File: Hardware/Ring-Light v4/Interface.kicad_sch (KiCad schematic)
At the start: 15 parts, among them J2 USB_B_Micro, U37 CP2102N-A02-GQFN20R

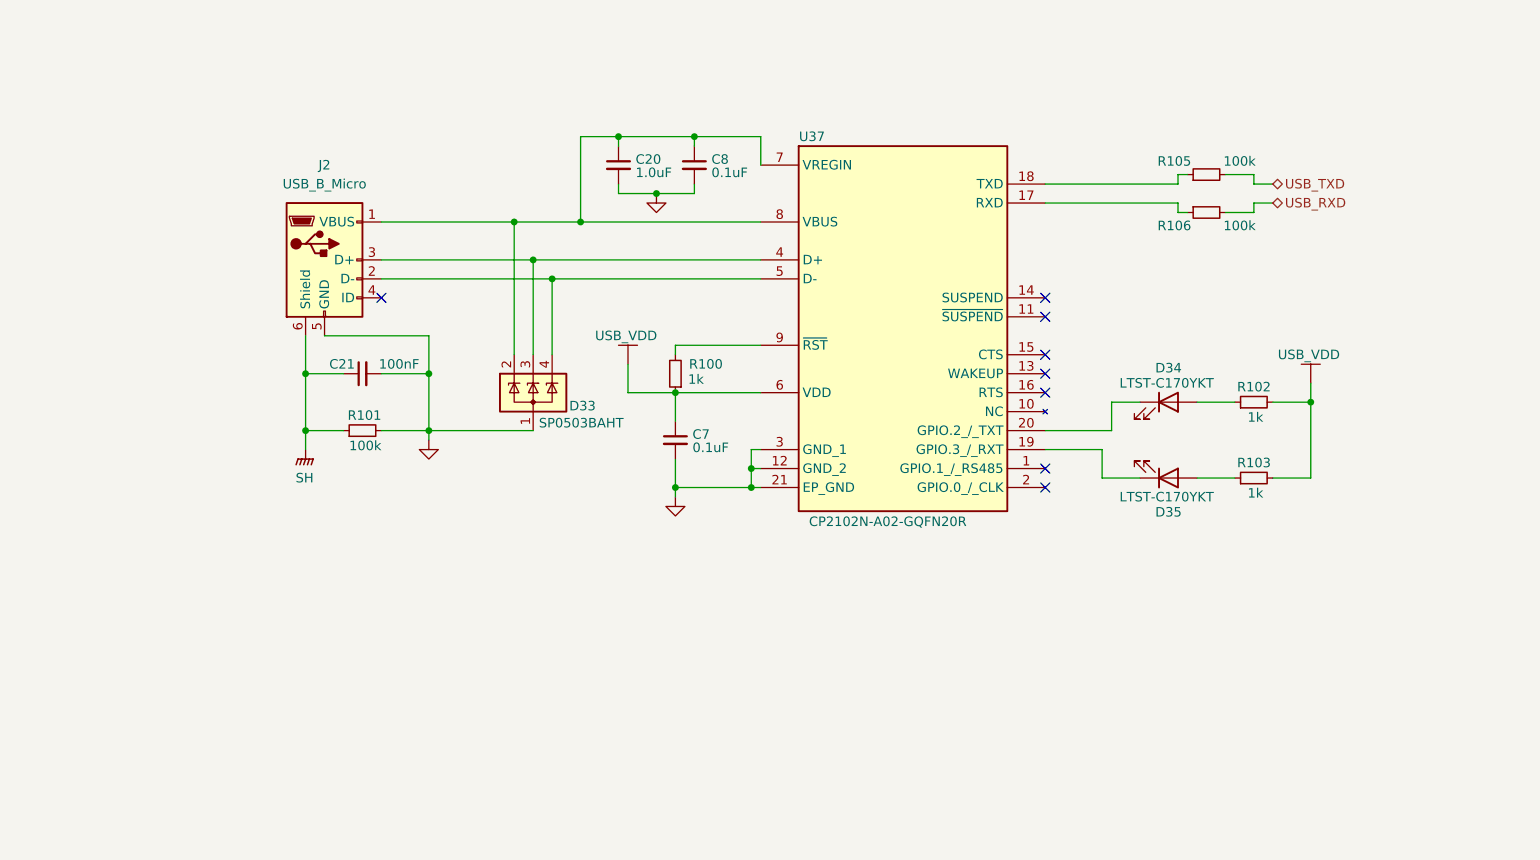
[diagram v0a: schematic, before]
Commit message: m
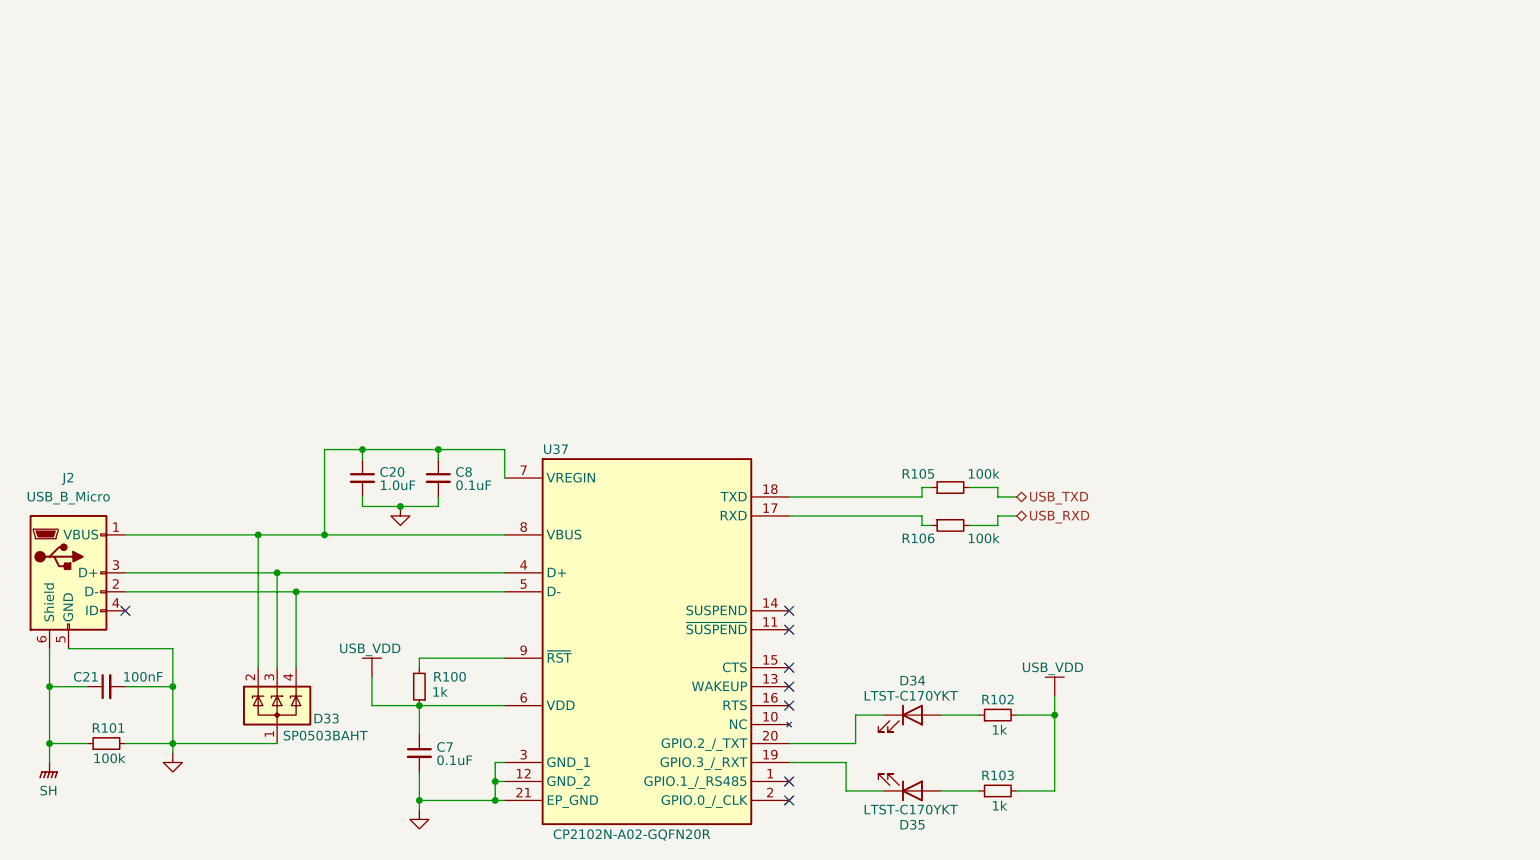
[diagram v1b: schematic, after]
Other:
- moved on the sheet: C20, C21, C7, C8, D33, D34, D35, J2, R100, R101, R102, R103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

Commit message: m
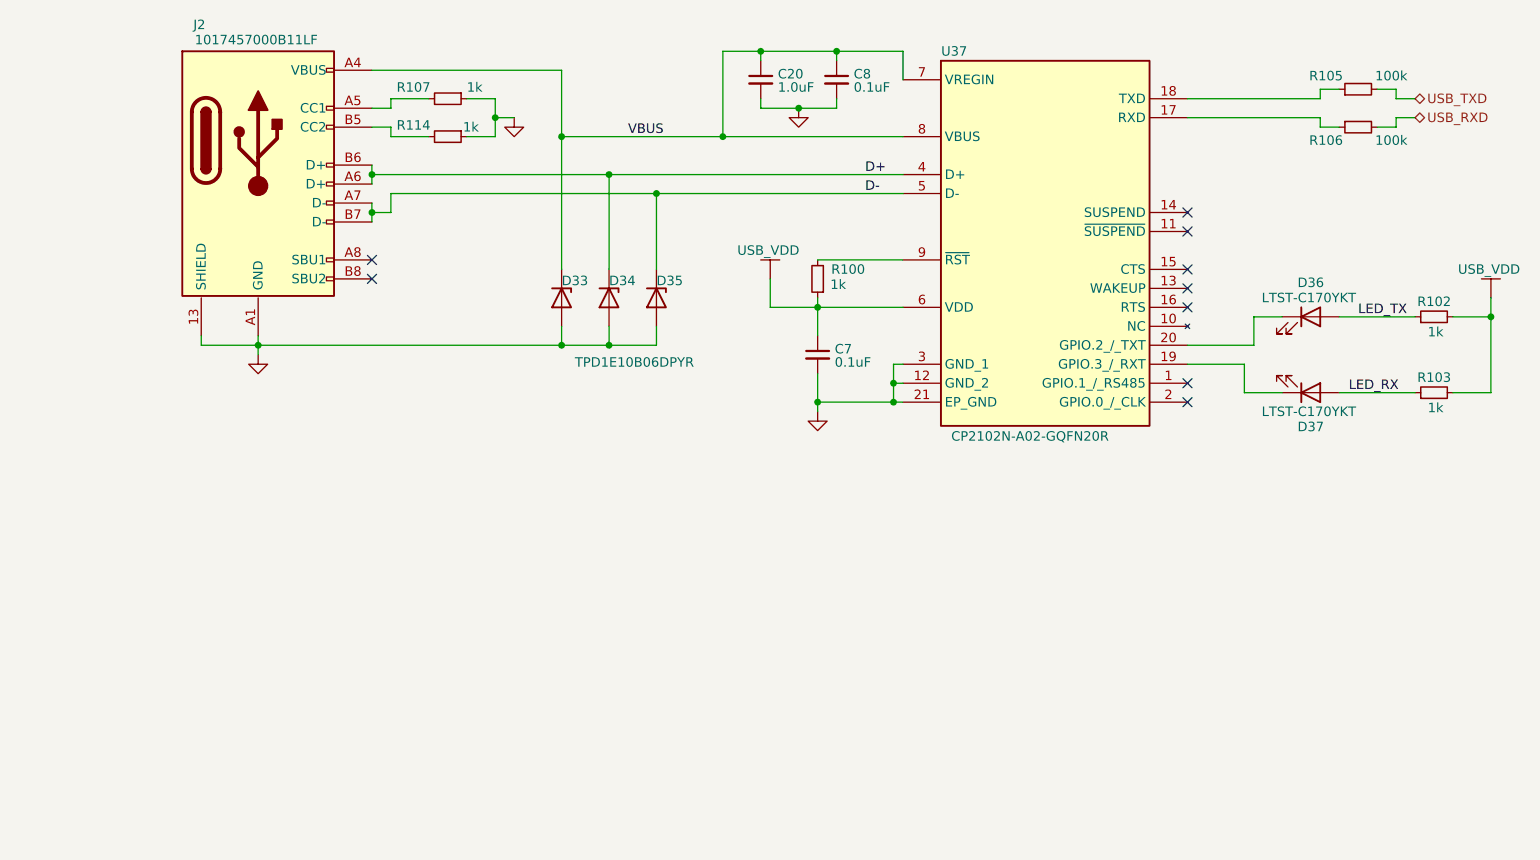
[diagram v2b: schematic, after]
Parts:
- removed C21: 100nF, Capacitor_SMD:C_0603_1608Metric, symbol Device:C_Small
- removed D33: SP0503BAHT, Package_TO_SOT_SMD:SOT-143, symbol Power_Protection:SP0503BAHT
- removed J2: USB_B_Micro, symbol Connector:USB_B_Micro
- removed R101: 100k, Resistor_SMD:R_0402_1005Metric, symbol Device:R_Small
- added D33, D34, D35: TPD1E10B06DPYR, Library:TPD1E10B06DPYR, symbol Diode:ESD5Zxx
- added J2: 1017457000B11LF, symbol Connector:USB_C_Receptacle
- added R107, R114: 1k, Resistor_SMD:R_0402_1005Metric, symbol Device:R_Small
- C20, C7, C8: footprint Capacitor_SMD:C_0603_1608Metric -> Capacitor_SMD:C_0402_1005Metric
- renumbered D34 to D36, D35 to D37
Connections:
- net GND: now also D33.2 (A), D34.2 (A), D35.2 (A), J2.13 (SHIELD), J2.A1 (GND), R107.1, R114.1
- net at C20.1, C8.1, U37.7 (VREGIN)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: no longer names the net of C20.1, C8.1, U37.7 (VREGIN), U37.8 (VBUS)
- net at C20.1, C8.1, U37.7 (VREGIN)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: now also D33.1 (K), J2.A4 (VBUS), J2.B4 (VBUS)
- net LED_RX: now reaches D37.3 (A), D37.4 (A), R103.1
- net D-: now reaches U37.5 (D-)
- net D-: now also D35.1 (K), J2.A7 (D-), J2.B7 (D-)
- net D+: now reaches U37.4 (D+)
- net D+: now also D34.1 (K), J2.A6 (D+), J2.B6 (D+)
- net LED_TX: now reaches D36.3 (A), D36.4 (A), R102.1
- new net: J2.B5 (CC2), R114.2
- new net: J2.A5 (CC1), R107.2
- new net: J2.14 (SHIELD), J2.15 (SHIELD), J2.16 (SHIELD)
- no-connect marks 8 -> 9
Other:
- moved on the sheet: C20, C7, C8, D36, D37, R100, R102, R103, R105, R106, U37
